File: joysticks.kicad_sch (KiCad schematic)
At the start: 27 parts, among them J1 DB9_Male_MountingHoles, J2 DB9_Male_MountingHoles, J25 Joystick Ports Mezannine Lower, J26 Joystick Ports Mezannine Upper, SW1 SW_Push_DPDT, U10 74LS06N, U11 74LS06N, U5 74LS06N, U6 74LVC374, U7 74LVC374, U8 74LS373, U9 74LS373

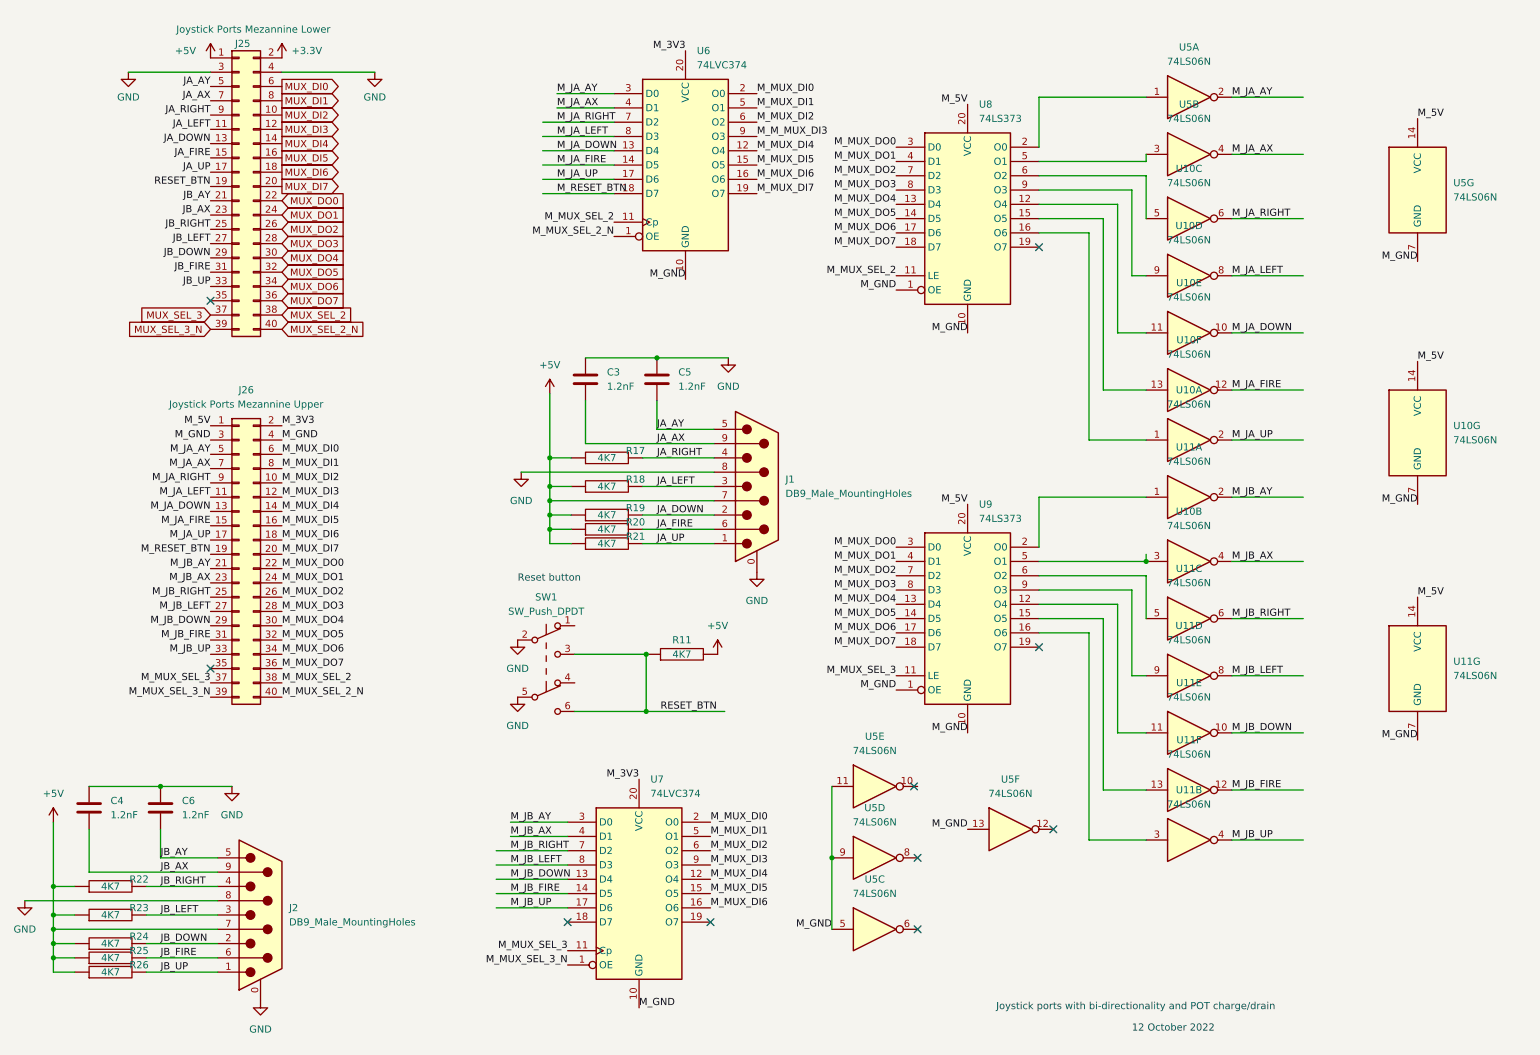
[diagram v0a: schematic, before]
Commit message: start routing joystick mezzannine
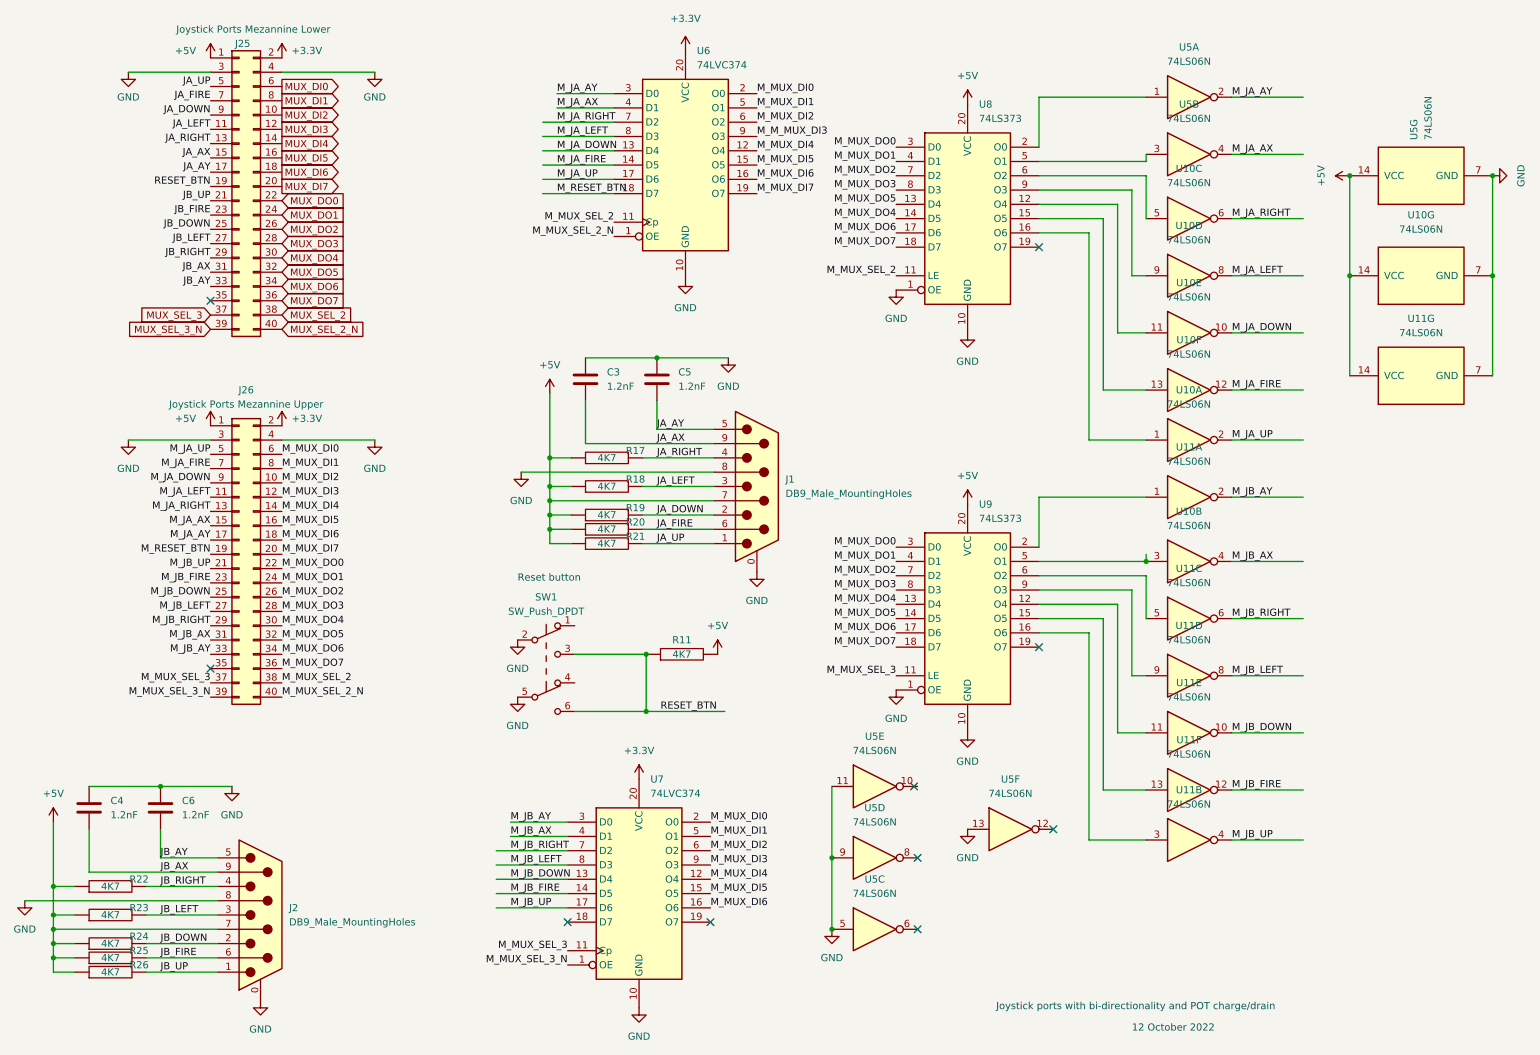
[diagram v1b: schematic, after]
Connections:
- net M_3V3 is gone; now on net +3V3: J26.2 (Pin_2), U6.20 (VCC), U7.20 (VCC)
- net M_5V is gone; now on net +5V: J26.1 (Pin_1), U10.14 (VCC), U11.14 (VCC), U5.14 (VCC), U8.20 (VCC), U9.20 (VCC)
- net M_GND is gone; now on net GND: J26.3 (Pin_3), J26.4 (Pin_4), U10.7 (GND), U11.7 (GND), U5.11, U5.13, U5.5, U5.7 (GND), U5.9, U6.10 (GND), U7.10 (GND), U8.1 (OE), U8.10 (GND), U9.1 (OE), U9.10 (GND)
- net JA_AX: now also J25.15 (Pin_15); no longer J25.7 (Pin_7)
- net JA_AY: now also J25.17 (Pin_17); no longer J25.5 (Pin_5)
- net JA_DOWN: now also J25.9 (Pin_9); no longer J25.13 (Pin_13)
- net JA_FIRE: now also J25.7 (Pin_7); no longer J25.15 (Pin_15)
- net JA_RIGHT: now also J25.13 (Pin_13); no longer J25.9 (Pin_9)
- net JA_UP: now also J25.5 (Pin_5); no longer J25.17 (Pin_17)
- net JB_AX: now also J25.31 (Pin_31); no longer J25.23 (Pin_23)
- net JB_AY: now also J25.33 (Pin_33); no longer J25.21 (Pin_21)
- net JB_DOWN: now also J25.25 (Pin_25); no longer J25.29 (Pin_29)
- net JB_FIRE: now also J25.23 (Pin_23); no longer J25.31 (Pin_31)
- net JB_RIGHT: now also J25.29 (Pin_29); no longer J25.25 (Pin_25)
- net JB_UP: now also J25.21 (Pin_21); no longer J25.33 (Pin_33)
- net M_JA_AX: now also J26.15 (Pin_15); no longer J26.7 (Pin_7)
- net M_JA_AY: now also J26.17 (Pin_17); no longer J26.5 (Pin_5)
- net M_JA_DOWN: now also J26.9 (Pin_9); no longer J26.13 (Pin_13)
- net M_JA_FIRE: now also J26.7 (Pin_7); no longer J26.15 (Pin_15)
- net M_JA_RIGHT: now also J26.13 (Pin_13); no longer J26.9 (Pin_9)
- net M_JA_UP: now also J26.5 (Pin_5); no longer J26.17 (Pin_17)
- net M_JB_AX: now also J26.31 (Pin_31); no longer J26.23 (Pin_23)
- net M_JB_AY: now also J26.33 (Pin_33); no longer J26.21 (Pin_21)
- net M_JB_DOWN: now also J26.25 (Pin_25); no longer J26.29 (Pin_29)
- net M_JB_FIRE: now also J26.23 (Pin_23); no longer J26.31 (Pin_31)
- net M_JB_RIGHT: now also J26.29 (Pin_29); no longer J26.25 (Pin_25)
- net M_JB_UP: now also J26.21 (Pin_21); no longer J26.33 (Pin_33)
- net M_MUX_DO4: now also U8.14 (D5); no longer U8.13 (D4)
- net M_MUX_DO5: now also U8.13 (D4); no longer U8.14 (D5)
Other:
- moved on the sheet: U10G, U11G, U5G
